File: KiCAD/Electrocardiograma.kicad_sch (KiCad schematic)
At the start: 93 parts, among them J1 54-00174, J2 Conn_01x02_Pin, J3 USB_C_Receptacle_PowerOnly_6P, J4 Conn_01x02_Pin, J5 Conn_01x02_Pin, J6 Conn_01x04_Pin, U1 INA823DT, U2 ESP32-C3-WROOM-02, U3 TLV1117-33, U4 TLV4888, U5 TLV4888, U6 TLV1117-ADJ, U7 SC6038, U8 CH224K

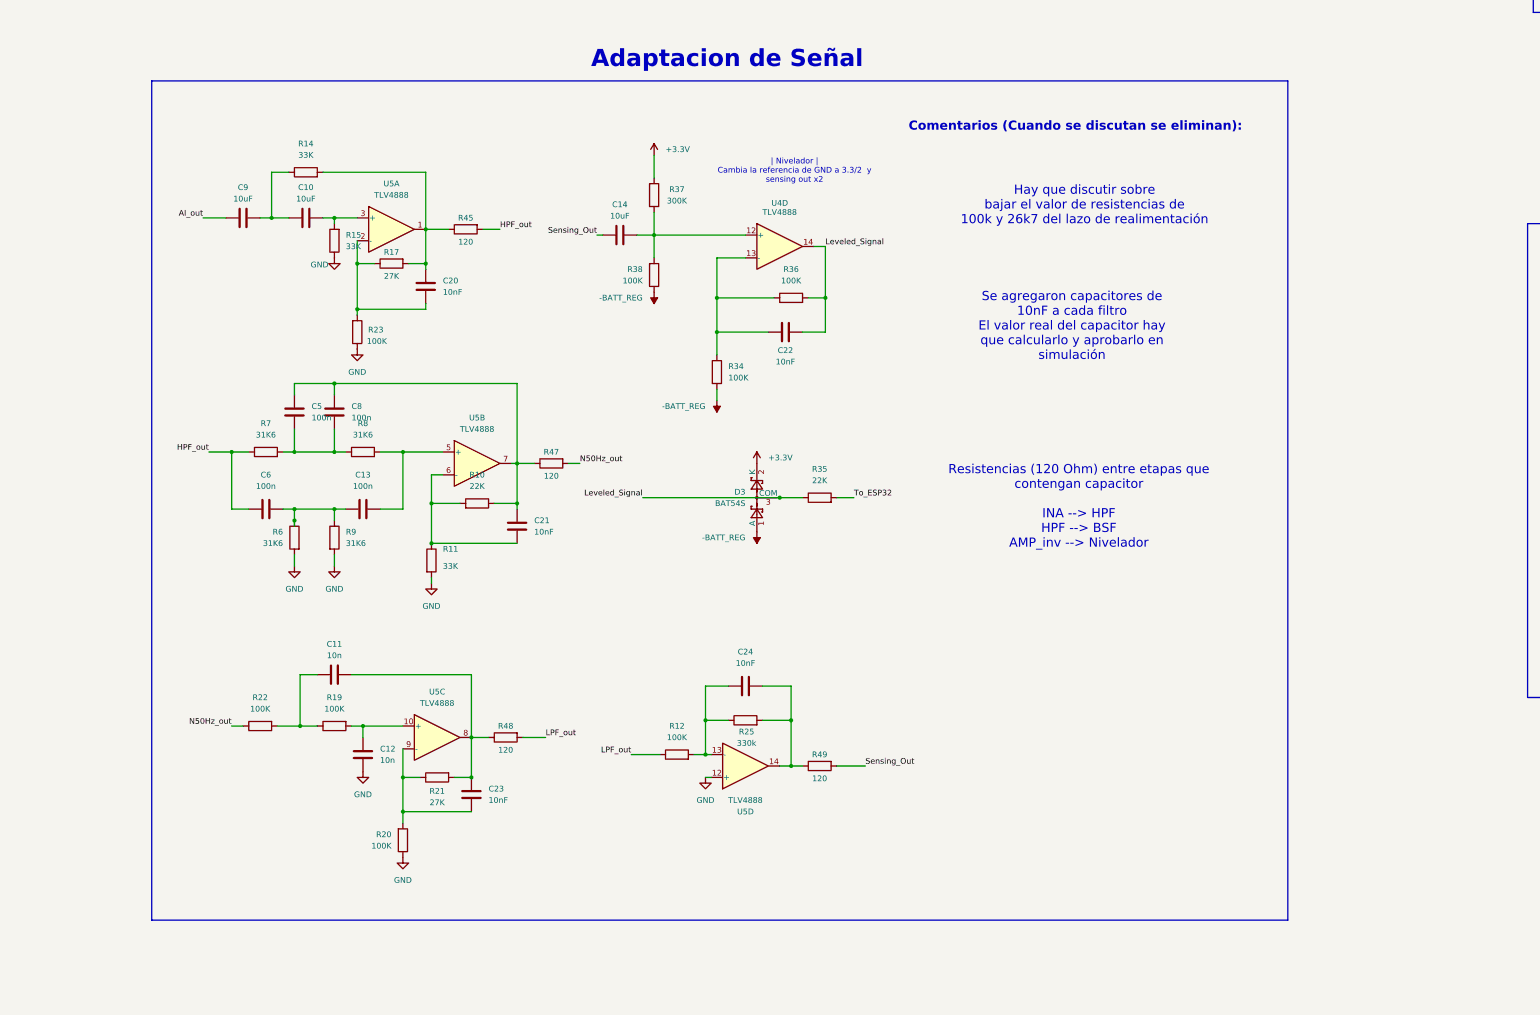
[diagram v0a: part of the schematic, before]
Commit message: diseño capacitores Cf
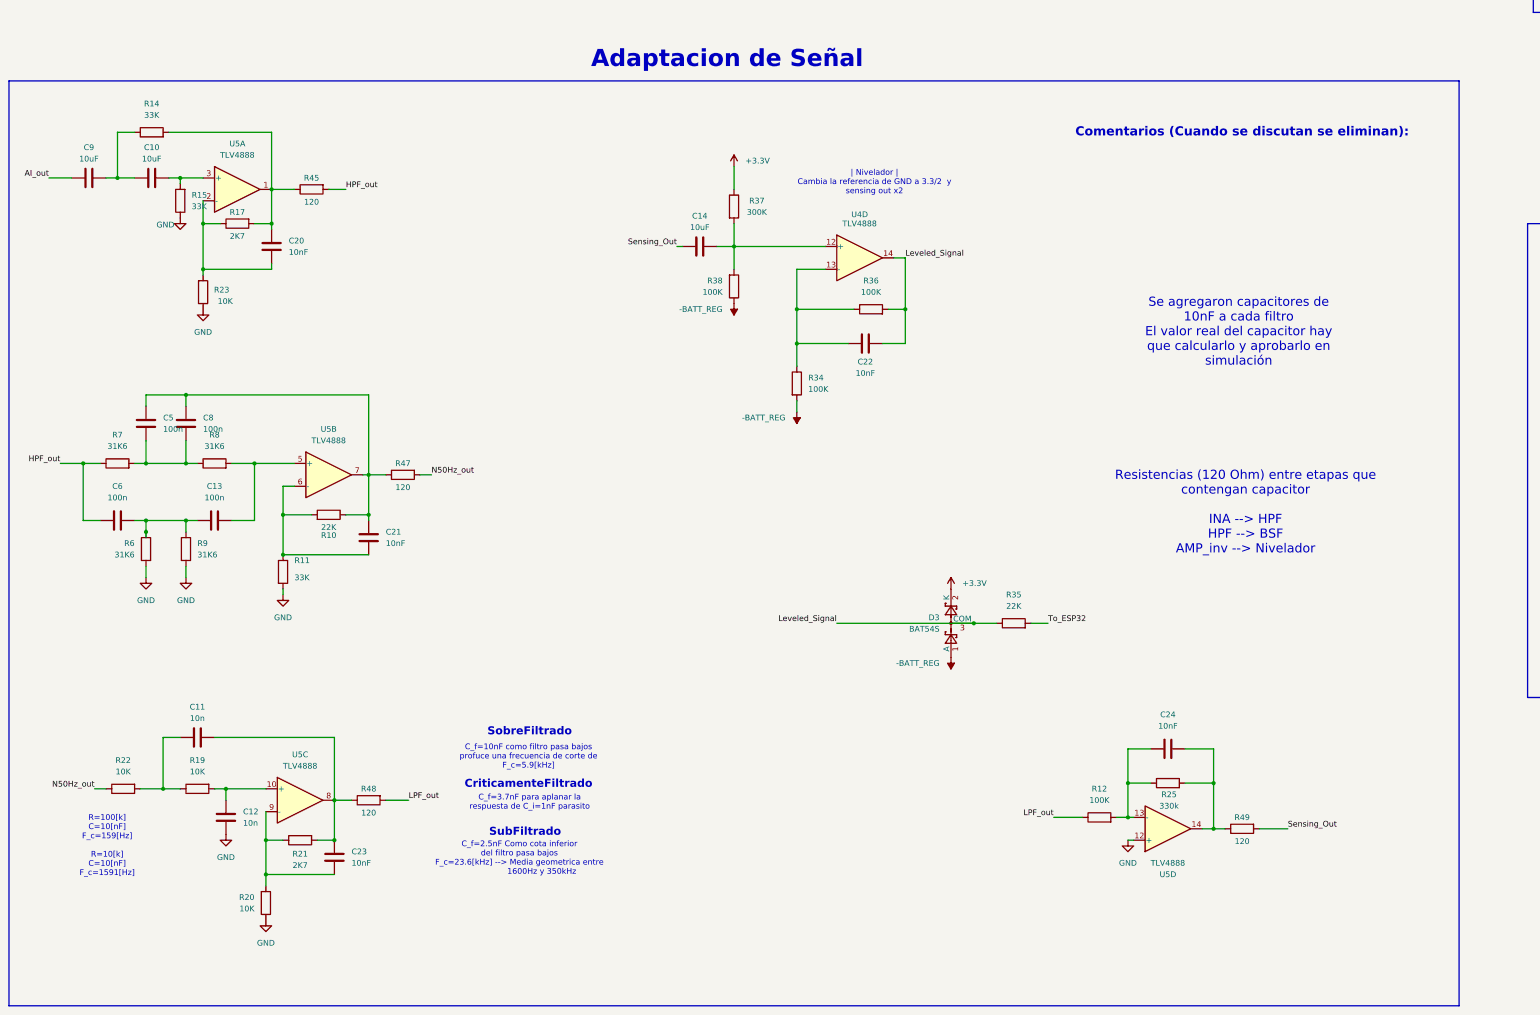
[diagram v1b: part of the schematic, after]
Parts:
- R17, R21: value 27K -> 2K7
- R19, R20, R22, R23: value 100K -> 10K
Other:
- note added: "C_f=10nF como filtro pasa bajos profuce una frecuencia de corte de F_c=5.9[kHz]"
- note added: "C_f=2.5nF Como cota inferior del filtro pasa bajos F_c=23.6[kHz] --> Media geometrica entre 1600Hz y 350kHz"
- note added: "C_f=3.7nF para aplanar la respuesta de C_i=1nF parasito"
- note added: "CriticamenteFiltrado"
- note added: "R=100[k] C=10[nF] F_c=159[Hz] R=10[k] C=10[nF] F_c=1591[Hz]"
- note added: "SobreFiltrado"
- note added: "SubFiltrado"
- note removed: "Hay que discutir sobre bajar el valor de resistencias de 100k y 26k7 del lazo de realimentación"
- moved on the sheet: C10, C11, C12, C13, C14, C20, C21, C22, C23, C24, C5, C6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
